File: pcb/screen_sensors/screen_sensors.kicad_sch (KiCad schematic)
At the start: 14 parts, among them J1 WAVESHARE_I2C, J2 BOILER_PROBE, J3 XDB401_ANALOG, U1 ADS1115IDGSR, U2 SHT40-AD1B

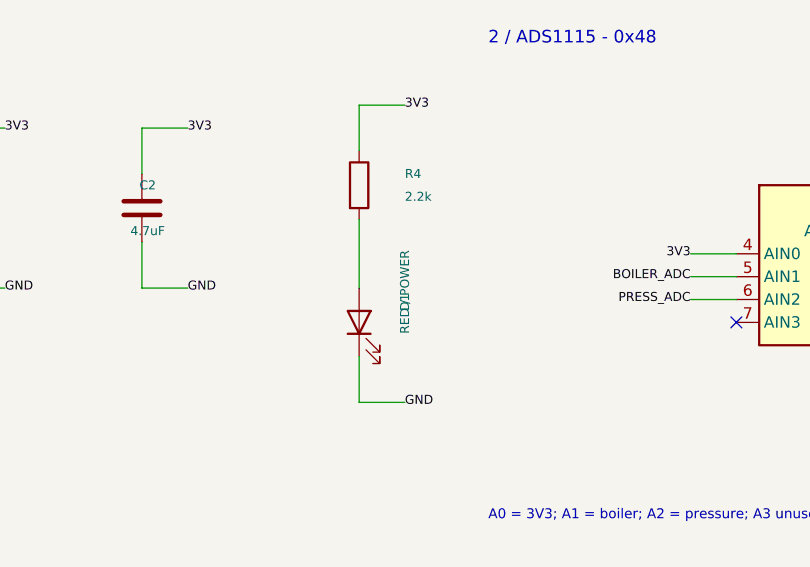
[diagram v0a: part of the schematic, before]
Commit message: Rename sensor PCB project and share manufacturing exporter
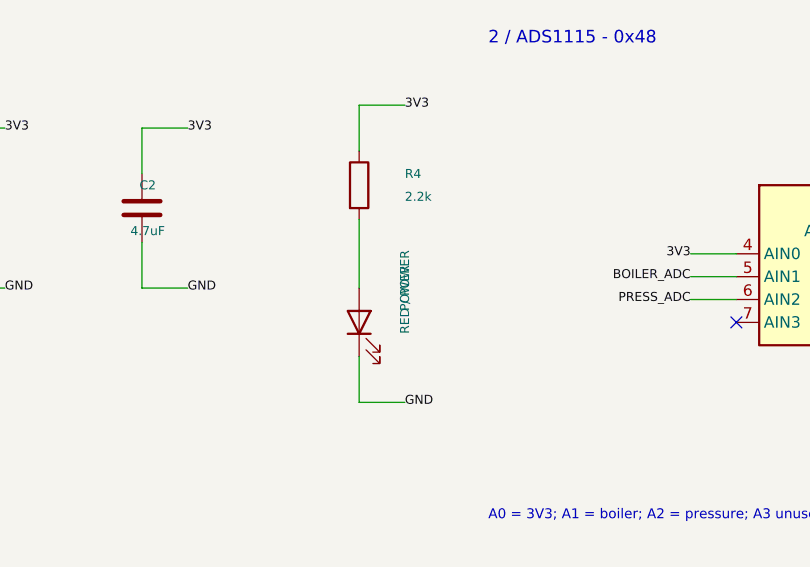
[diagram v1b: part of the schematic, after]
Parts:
- renumbered D1 to POWER
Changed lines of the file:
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@@
 (pin "3")
 (pin "4")
-(instances (project "screen_sensors_draft" (path "/b733619e-0a21-4de7-9d63-5b29c9c92157" (reference "J1") (unit 1)))) )
+(instances (project "screen_sensors" (path "/b733619e-0a21-4de7-9d63-5b29c9c92157" (reference "J1") (unit 1)))) )
 (wire (pts (xy 76.2 46.99) (xy 76.2 41.91)) (stroke (width 0) (type default)))
 (wire (pts (xy 76.2 41.91) (xy 81.28 41.91)) (stroke (width 0) (type default)))
@@
 (pin "1")
 (pin "2")
-(instances (project "screen_sensors_draft" (path "/b733619e-0a21-4de7-9d63-5b29c9c92157" (reference "C1") (unit 1)))) )
+(instances (project "screen_sensors" (path "/b733619e-0a21-4de7-9d63-5b29c9c92157" (reference "C1") (unit 1)))) )
 (wire (pts (xy 96.52 46.99) (xy 96.52 41.91)) (stroke (width 0) (type default)))
 (wire (pts (xy 96.52 41.91) (xy 101.6 41.91)) (stroke (width 0) (type default)))
@@
 (pin "1")
 (pin "2")
-(instances (project "screen_sensors_draft" (path "/b733619e-0a21-4de7-9d63-5b29c9c92157" (reference "C2") (unit 1)))) )
+(instances (project "screen_sensors" (path "/b733619e-0a21-4de7-9d63-5b29c9c92157" (reference "C2") (unit 1)))) )
 (wire (pts (xy 25.4 73.66) (xy 25.4 78.74)) (stroke (width 0) (type default)))
 (wire (pts (xy 25.4 78.74) (xy 30.48 78.74)) (stroke (width 0) (type default)))
@@
 (property "Datasheet" "" (at 25.4 73.66 0) (effects (font (size 1.0 1.0)) (hide yes)))
 (pin "1")
-(instances (project "screen_sensors_draft" (path "/b733619e-0a21-4de7-9d63-5b29c9c92157" (reference "#FLG01") (unit 1)))) )
+(instances (project "screen_sensors" (path "/b733619e-0a21-4de7-9d63-5b29c9c92157" (reference "#FLG01") (unit 1)))) )
 (wire (pts (xy 48.26 73.66) (xy 48.26 78.74)) (stroke (width 0) (type default)))
 (wire (pts (xy 48.26 78.74) (xy 53.34 78.74)) (stroke (width 0) (type default)))
@@
 (property "Datasheet" "" (at 48.26 73.66 0) (effects (font (size 1.0 1.0)) (hide yes)))
 (pin "1")
-(instances (project "screen_sensors_draft" (path "/b733619e-0a21-4de7-9d63-5b29c9c92157" (reference "#FLG02") (unit 1)))) )
+(instances (project "screen_sensors" (path "/b733619e-0a21-4de7-9d63-5b29c9c92157" (reference "#FLG02") (unit 1)))) )
 (text "No added I2C pull-ups: Waveshare H7 already has 4.7k." (at 20 85 0) (effects (font (size 1.1 1.1)) (justify left)))
 (text "2 / ADS1115 - 0x48" (at 135 32 0) (effects (font (size 1.4 1.4)) (justify left)))
@@
 (pin "9")
 (pin "10")
-(instances (project "screen_sensors_draft" (path "/b733619e-0a21-4de7-9d63-5b29c9c92157" (reference "U1") (unit 1)))) )
+(instances (project "screen_sensors" (path "/b733619e-0a21-4de7-9d63-5b29c9c92157" (reference "U1") (unit 1)))) )
 (text "A0 = 3V3; A1 = boiler; A2 = pressure; A3 unused." (at 135 85 0) (effects (font (size 1.1 1.1)) (justify left)))
 (text "3 / Boiler NTC or PT1000" (at 20 98 0) (effects (font (size 1.4 1.4)) (justify left)))
@@
 (pin "1")
 (pin "2")
-(instances (project "screen_sensors_draft" (path "/b733619e-0a21-4de7-9d63-5b29c9c92157" (reference "J2") (unit 1)))) )
+(instances (project "screen_sensors" (path "/b733619e-0a21-4de7-9d63-5b29c9c92157" (reference "J2") (unit 1)))) )
 (wire (pts (xy 73.66 113.03) (xy 73.66 107.95)) (stroke (width 0) (type default)))
 (wire (pts (xy 73.66 107.95) (xy 78.74 107.95)) (stroke (width 0) (type default)))
@@
 (pin "1")
 (pin "2")
-(instances (project "screen_sensors_draft" (path "/b733619e-0a21-4de7-9d63-5b29c9c92157" (reference "R1") (unit 1)))) )
+(instances (project "screen_sensors" (path "/b733619e-0a21-4de7-9d63-5b29c9c92157" (reference "R1") (unit 1)))) )
 (text "Probe between 3V3 and DIV. Fixed resistor from DIV to GND." (at 20 135 0) (effects (font (size 1.1 1.1)) (justify left)))
 (text "Rprobe = R1 * (A0/A1 - 1). Use new-board calibration." (at 20 141 0) (effects (font (size 1.1 1.1)) (justify left)))
@@
 (pin "2")
 (pin "3")
-(instances (project "screen_sensors_draft" (path "/b733619e-0a21-4de7-9d63-5b29c9c92157" (reference "J3") (unit 1)))) )
+(instances (project "screen_sensors" (path "/b733619e-0a21-4de7-9d63-5b29c9c92157" (reference "J3") (unit 1)))) )
 (wire (pts (xy 208.28 113.03) (xy 208.28 107.95)) (stroke (width 0) (type default)))
 (wire (pts (xy 208.28 107.95) (xy 213.36 107.95)) (stroke (width 0) (type default)))
@@
 (pin "1")
 (pin "2")
-(instances (project "screen_sensors_draft" (path "/b733619e-0a21-4de7-9d63-5b29c9c92157" (reference "R3") (unit 1)))) )
+(instances (project "screen_sensors" (path "/b733619e-0a21-4de7-9d63-5b29c9c92157" (reference "R3") (unit 1)))) )
 (wire (pts (xy 233.68 113.03) (xy 233.68 107.95)) (stroke (width 0) (type default)))
 (wire (pts (xy 233.68 107.95) (xy 238.76 107.95)) (stroke (width 0) (type default)))
@@
 (pin "1")
 (pin "2")
-(instances (project "screen_sensors_draft" (path "/b733619e-0a21-4de7-9d63-5b29c9c92157" (reference "C3") (unit 1)))) )
+(instances (project "screen_sensors" (path "/b733619e-0a21-4de7-9d63-5b29c9c92157" (reference "C3") (unit 1)))) )
 (wire (pts (xy 259.08 113.03) (xy 259.08 107.95)) (stroke (width 0) (type default)))
 (wire (pts (xy 259.08 107.95) (xy 264.16 107.95)) (stroke (width 0) (type default)))
@@
 (pin "1")
 (pin "2")
-(instances (project "screen_sensors_draft" (path "/b733619e-0a21-4de7-9d63-5b29c9c92157" (reference "C4") (unit 1)))) )
+(instances (project "screen_sensors" (path "/b733619e-0a21-4de7-9d63-5b29c9c92157" (reference "C4") (unit 1)))) )
 (text "No voltage divider / amplifier needed. Pressure = 6*(Vout-0.4) bar nominal." (at 155 135 0) (effects (font (size 1.1 1.1)) (justify left)))
 (text "Verify supply current, output impedance, startup and ratiometry before manufacture." (at 155 141 0) (effects (font (size 1.1 1.1)) (justify left)))
@@
 (pin "3")
 (pin "4")
-(instances (project "screen_sensors_draft" (path "/b733619e-0a21-4de7-9d63-5b29c9c92157" (reference "U2") (unit 1)))) )
+(instances (project "screen_sensors" (path "/b733619e-0a21-4de7-9d63-5b29c9c92157" (reference "U2") (unit 1)))) )
 (wire (pts (xy 83.82 171.45) (xy 83.82 166.37)) (stroke (width 0) (type default)))
 (wire (pts (xy 83.82 166.37) (xy 88.9 166.37)) (stroke (width 0) (type default)))
@@
 (pin "1")
 (pin "2")
-(instances (project "screen_sensors_draft" (path "/b733619e-0a21-4de7-9d63-5b29c9c92157" (reference "C5") (unit 1)))) )
+(instances (project "screen_sensors" (path "/b733619e-0a21-4de7-9d63-5b29c9c92157" (reference "C5") (unit 1)))) )
 (text "Place near board edge, exposed to box air, away from display heat." (at 20 194 0) (effects (font (size 1.1 1.1)) (justify left)))
 (text "Humidity sensor opening must remain free of flux, coating and adhesives." (at 20 200 0) (effects (font (size 1.1 1.1)) (justify left)))
@@
 (pin "1")
 (pin "2")
-(instances (project "screen_sensors_draft" (path "/b733619e-0a21-4de7-9d63-5b29c9c92157" (reference "R4") (unit 1)))) )
+(instances (project "screen_sensors" (path "/b733619e-0a21-4de7-9d63-5b29c9c92157" (reference "R4") (unit 1)))) )
 (symbol (lib_id "Device:LED") (at 120.65 63.5 90) (unit 1) (in_bom yes) (on_board yes) (dnp no)
-(property "Reference" "D1" (at 125.73 62.23 0) (effects (font (size 1.0 1.0)) (justify left)))
+(property "Reference" "POWER" (at 125.73 62.23 0) (effects (font (size 1.0 1.0)) (justify left)))
 (property "Value" "RED / POWER" (at 125.73 64.77 0) (effects (font (size 1.0 1.0)) (justify left)))
 (property "Footprint" "LED_SMD:LED_0603_1608Metric" (at 120.65 63.5 0) (effects (font (size 1.0 1.0)) (hide yes)))
@@
 (pin "1")
 (pin "2")
-(instances (project "screen_sensors_draft" (path "/b733619e-0a21-4de7-9d63-5b29c9c92157" (reference "D1") (unit 1)))) )
+(instances (project "screen_sensors" (path "/b733619e-0a21-4de7-9d63-5b29c9c92157" (reference "POWER") (unit 1)))) )
 (text "POWER: 3V3 present; does not verify I2C communication." (at 20 84 0) (effects (font (size 1.1 1.1)) (justify left)))
 (sheet_instances (path "/" (page "1"))) (embedded_fonts no))
